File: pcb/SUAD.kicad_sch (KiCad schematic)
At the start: 14 parts, among them Q1 AO3401A, Q2 AO3401A, Q3 AO3401A, U1 Pico

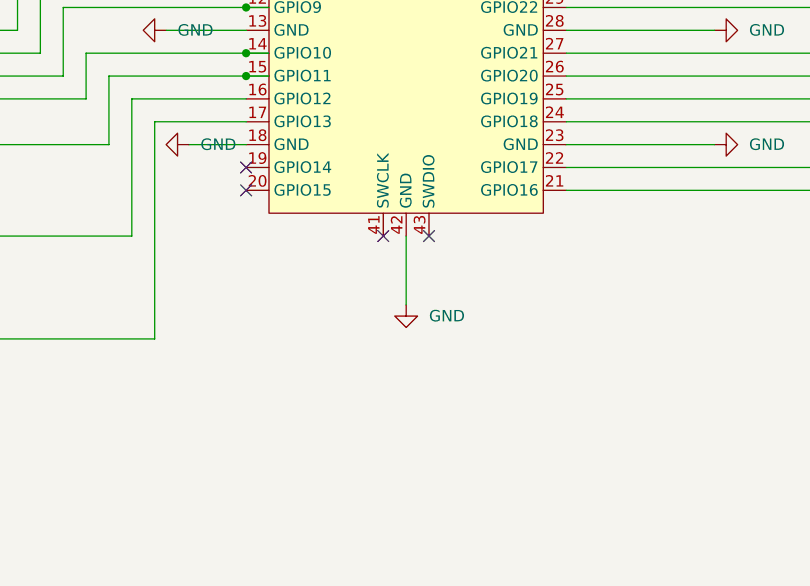
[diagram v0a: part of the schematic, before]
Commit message: Routed
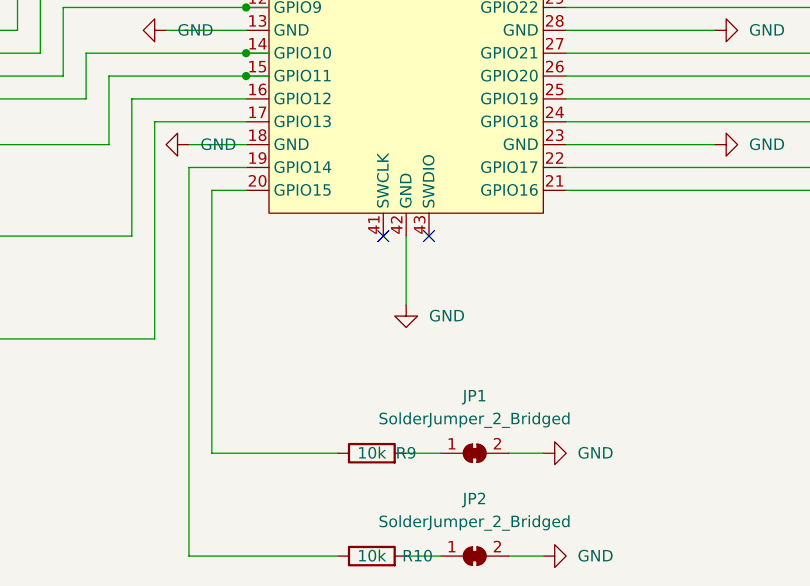
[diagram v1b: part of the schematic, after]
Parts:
- added JP1, JP2: SolderJumper_2_Bridged, Jumper:SolderJumper-2_P1.3mm_Bridged_RoundedPad1.0x1.5mm, symbol Jumper:SolderJumper_2_Bridged
- added R10, R9: 10k, Resistor_SMD:R_0603_1608Metric, symbol Device:R
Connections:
- net GND: now also JP1.2 (B), JP2.2 (B)
- net at U1.19 (GPIO14): now also R10.1
- net at U1.20 (GPIO15): now also R9.1
- new net: JP1.1 (A), R9.2
- new net: JP2.1 (A), R10.2
- no-connect marks 10 -> 8

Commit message: Fixed ERC and DRC
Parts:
- DS1: LCSC (none) -> C226010
- Q1, Q2, Q3: LCSC (none) -> C15127
- R1, R2, R3, R4, R5, R6, R7, R8: LCSC (none) -> C23138
- R10, R9: LCSC (none) -> C25804
- RV1: LCSC (none) -> C470765
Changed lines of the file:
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@@
+      (effects (font (size 1.27 1.27)) hide)
+    )
+    (property "LCSC" "C23138" (id 4) (at 95.25 92.71 0)
       (effects (font (size 1.27 1.27)) hide)
     )
@@
       (effects (font (size 1.27 1.27)) (justify left) hide)
     )
+    (property "LCSC" "C15127" (id 4) (at 60.96 115.57 0)
+      (effects (font (size 1.27 1.27)) hide)
+    )
     (pin "1")
     (pin "2")
@@
       (effects (font (size 1.27 1.27)) hide)
     )
+    (property "LCSC" "C23138" (id 4) (at 95.25 95.25 0)
+      (effects (font (size 1.27 1.27)) hide)
+    )
     (pin "1")
     (pin "2")
@@
       (effects (font (size 1.27 1.27)) hide)
     )
+    (property "LCSC" "C25804" (id 4) (at 152.4 149.86 0)
+      (effects (font (size 1.27 1.27)) hide)
+    )
     (pin "1")
     (pin "2")
@@
       (effects (font (size 1.27 1.27)) hide)
     )
+    (property "LCSC" "C23138" (id 4) (at 95.25 105.41 0)
+      (effects (font (size 1.27 1.27)) hide)
+    )
     (pin "1")
     (pin "2")
@@
       (effects (font (size 1.27 1.27)) (justify left) hide)
     )
+    (property "LCSC" "C15127" (id 4) (at 45.72 125.73 0)
+      (effects (font (size 1.27 1.27)) hide)
+    )
     (pin "1")
     (pin "2")
@@
     (property "Datasheet" "http://www.aosmd.com/pdfs/datasheet/AO3401A.pdf" (id 3) (at 29.21 137.16 0)
       (effects (font (size 1.27 1.27)) (justify left) hide)
+    )
+    (property "LCSC" "C15127" (id 4) (at 29.21 137.16 0)
+      (effects (font (size 1.27 1.27)) hide)
     )
     (pin "1")
@@
       (effects (font (size 1.27 1.27)) hide)
     )
+    (property "LCSC" "C23138" (id 4) (at 95.25 102.87 0)
+      (effects (font (size 1.27 1.27)) hide)
+    )
     (pin "1")
     (pin "2")
@@
     )
     (property "Datasheet" "~" (id 3) (at 210.82 67.31 0)
+      (effects (font (size 1.27 1.27)) hide)
+    )
+    (property "LCSC" "C470765" (id 4) (at 210.82 67.31 0)
       (effects (font (size 1.27 1.27)) hide)
     )
@@
       (effects (font (size 1.27 1.27)) hide)
     )
+    (property "LCSC" "C23138" (id 4) (at 95.25 97.79 0)
+      (effects (font (size 1.27 1.27)) hide)
+    )
     (pin "1")
     (pin "2")
@@
       (effects (font (size 1.27 1.27)) hide)
     )
+    (property "LCSC" "C23138" (id 4) (at 95.25 100.33 0)
+      (effects (font (size 1.27 1.27)) hide)
+    )
     (pin "1")
     (pin "2")
@@
       (effects (font (size 1.27 1.27)) hide)
     )
+    (property "LCSC" "C23138" (id 4) (at 95.25 110.49 0)
+      (effects (font (size 1.27 1.27)) hide)
+    )
     (pin "1")
     (pin "2")
@@
     )
     (property "Datasheet" "" (id 3) (at 77.47 102.87 0)
+      (effects (font (size 1.27 1.27)) hide)
+    )
+    (property "LCSC" "C226010" (id 4) (at 74.93 101.6 0)
       (effects (font (size 1.27 1.27)) hide)
     )
@@
       (effects (font (size 1.27 1.27)) hide)
     )
+    (property "LCSC" "C25804" (id 4) (at 152.4 161.29 0)
+      (effects (font (size 1.27 1.27)) hide)
+    )
     (pin "1")
     (pin "2")
@@
       (effects (font (size 1.27 1.27)) hide)
     )
+    (property "LCSC" "C23138" (id 4) (at 95.25 107.95 0)
+      (effects (font (size 1.27 1.27)) hide)
+    )
